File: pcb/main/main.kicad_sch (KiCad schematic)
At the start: 4 parts

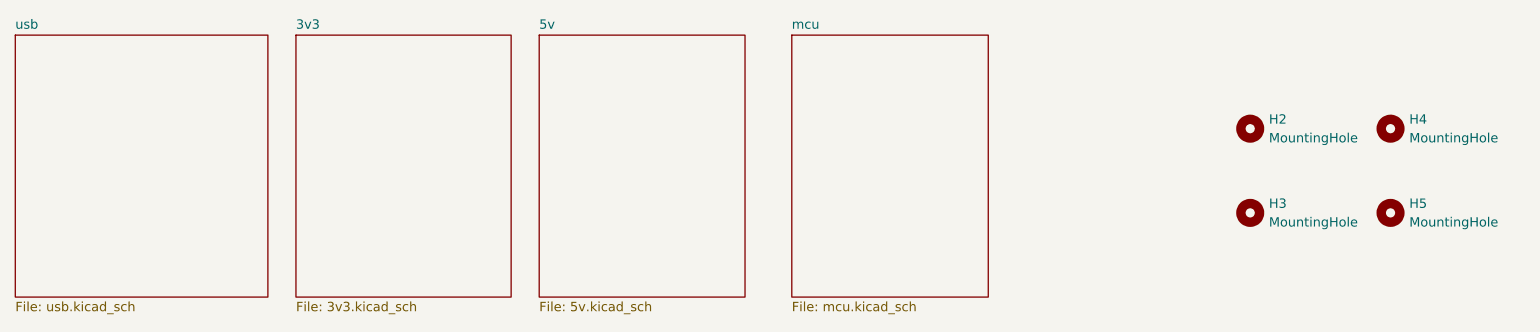
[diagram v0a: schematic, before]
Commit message: Rev B RC1
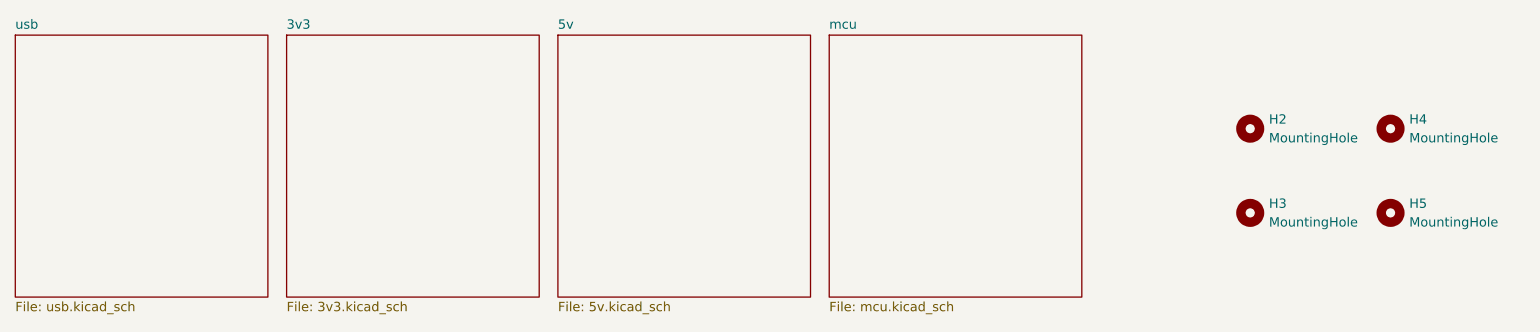
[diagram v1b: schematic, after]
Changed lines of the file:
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@@
 	)
 	(sheet
-		(at 148.59 38.1)
-		(size 26.67 35.56)
+		(at 153.67 38.1)
+		(size 34.29 35.56)
 		(exclude_from_sim no)
 		(in_bom yes)
@@
 		)
 		(property "Sheetname" "mcu"
-			(at 148.59 37.3884 0)
+			(at 153.67 37.3884 0)
 			(effects
 				(font
@@
 		)
 		(property "Sheetfile" "mcu.kicad_sch"
-			(at 148.59 74.2446 0)
+			(at 153.67 74.2446 0)
 			(effects
 				(font
@@
 	)
 	(sheet
-		(at 81.28 38.1)
-		(size 29.21 35.56)
+		(at 80.01 38.1)
+		(size 34.29 35.56)
 		(exclude_from_sim no)
 		(in_bom yes)
@@
 		)
 		(property "Sheetname" "3v3"
-			(at 81.28 37.3884 0)
+			(at 80.01 37.3884 0)
 			(effects
 				(font
@@
 		)
 		(property "Sheetfile" "3v3.kicad_sch"
-			(at 81.28 74.2446 0)
+			(at 80.01 74.2446 0)
 			(effects
 				(font
@@
 	)
 	(sheet
-		(at 114.3 38.1)
-		(size 27.94 35.56)
+		(at 116.84 38.1)
+		(size 34.29 35.56)
 		(exclude_from_sim no)
 		(in_bom yes)
@@
 		)
 		(property "Sheetname" "5v"
-			(at 114.3 37.3884 0)
+			(at 116.84 37.3884 0)
 			(effects
 				(font
@@
 		)
 		(property "Sheetfile" "5v.kicad_sch"
-			(at 114.3 74.2446 0)
+			(at 116.84 74.2446 0)
 			(effects
 				(font
